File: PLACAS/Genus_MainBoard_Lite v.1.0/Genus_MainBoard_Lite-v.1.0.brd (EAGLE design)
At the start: 70 x 86 mm, 60 parts, among them U1 FT232RLSSOP, U2 MP2307DN-LF-Z, X1 53398-06, X15 JST-XH-05-PIN-LONG-PAD, X2 JST-XH-08-PIN-ROUND-PAD, X3 USB-SMD-NS, X5 53398-06

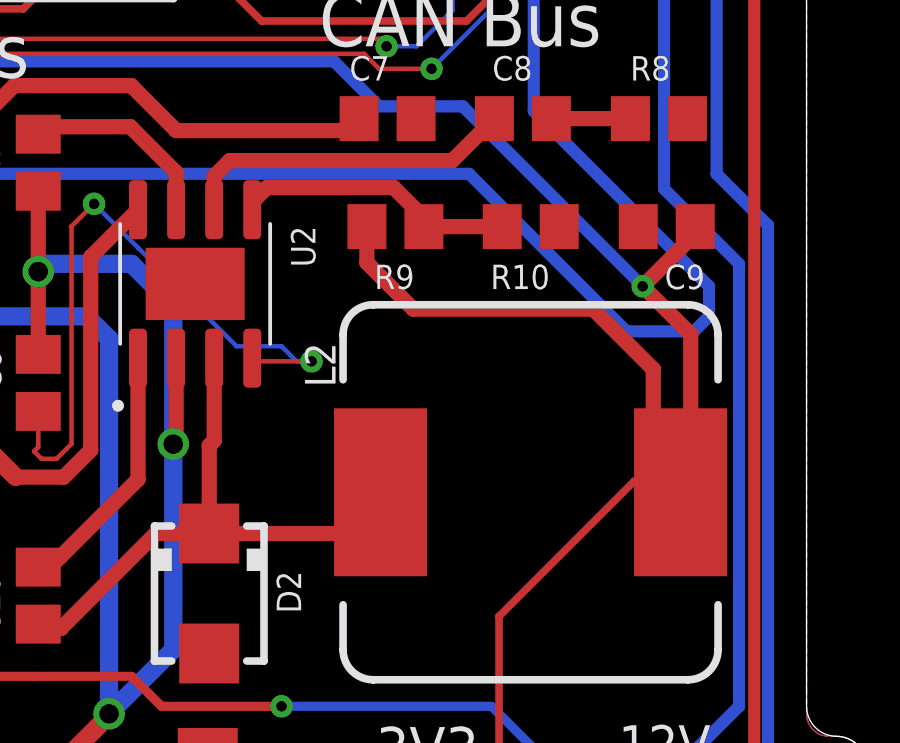
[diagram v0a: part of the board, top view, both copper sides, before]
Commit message: Add files via upload
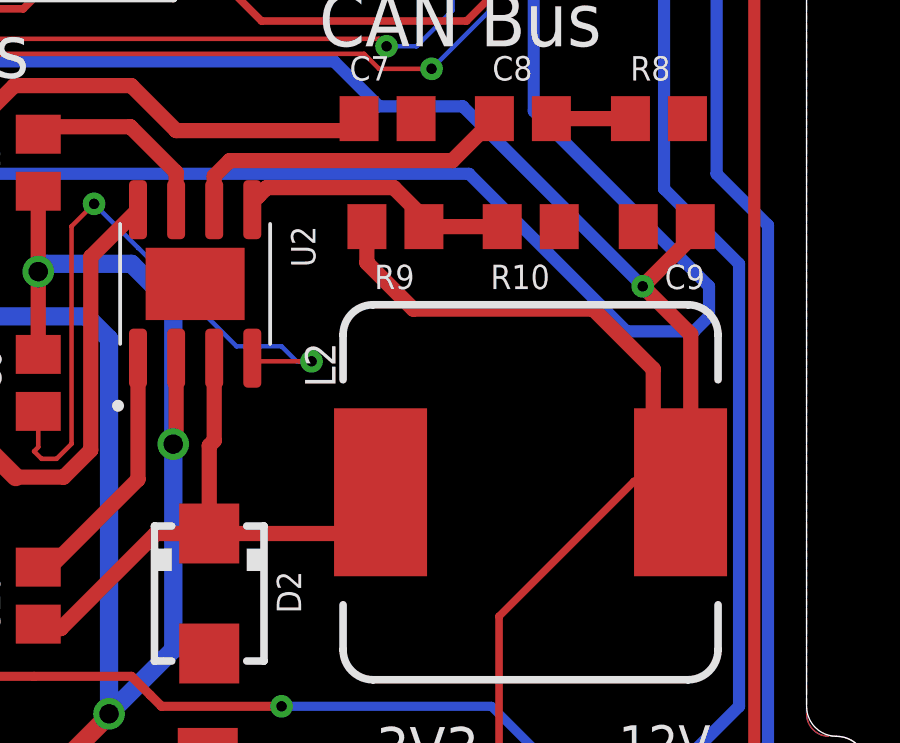
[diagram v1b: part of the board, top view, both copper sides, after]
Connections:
- new net BOOT: SLOT-1.A13, SLOT-2.A13
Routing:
- net OUT_3V3: track 86.4 -> 90.7 mm
- net N$12: track 22.1 -> 23.4 mm
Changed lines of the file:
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@@
 <?xml version="1.0" encoding="utf-8"?>
 <!DOCTYPE eagle SYSTEM "eagle.dtd">
-<eagle version="9.5.2">
+<eagle version="9.4.2">
 <drawing>
 <settings>
-<setting alwaysvectorfont="no"/>
+<setting alwaysvectorfont="yes"/>
 <setting verticaltext="up"/>
 </settings>
@@
 <contactref element="C10" pad="1"/>
 <contactref element="D2" pad="C"/>
-<wire x1="53.72" y1="26.73" x2="53.085" y2="26.095" width="0.6096" layer="1"/>
+<wire x1="53.085" y1="26.095" x2="53.72" y2="26.73" width="0.6096" layer="1"/>
 <wire x1="53.165" y1="27.5" x2="53.8" y2="28.135" width="0.508" layer="1"/>
 <wire x1="42.39" y1="23.74" x2="42.54" y2="23.59" width="0.508" layer="1"/>
@@
 <wire x1="46.31" y1="26.76" x2="48.09" y2="26.76" width="0.508" layer="1"/>
 <wire x1="43.14" y1="23.59" x2="46.31" y2="26.76" width="0.508" layer="1"/>
-<wire x1="48.09" y1="26.76" x2="53.66" y2="26.76" width="0.508" layer="1"/>
-<wire x1="53.66" y1="26.76" x2="54.14" y2="27.24" width="0.508" layer="1"/>
-<wire x1="53.8" y1="27.58" x2="53.8" y2="28.135" width="0.508" layer="1"/>
-<wire x1="54.14" y1="27.24" x2="53.8" y2="27.58" width="0.508" layer="1"/>
+<wire x1="52.5" y1="26.76" x2="48.09" y2="26.76" width="0.508" layer="1"/>
 <wire x1="48.09" y1="26.76" x2="48.09" y2="29.69" width="0.508" layer="1"/>
 <wire x1="48.255" y1="29.855" x2="48.255" y2="32.605" width="0.508" layer="1"/>
 <wire x1="48.09" y1="29.69" x2="48.255" y2="29.855" width="0.508" layer="1"/>
-<wire x1="53.165" y1="27.5" x2="53.72" y2="26.73" width="0" layer="19" extent="1-1"/>
+<wire x1="53.8" y1="28.135" x2="53.8" y2="28.06" width="0.1524" layer="1"/>
+<wire x1="53.8" y1="28.06" x2="52.5" y2="26.76" width="0.1524" layer="1"/>
+<wire x1="53.8" y1="28.135" x2="53.8" y2="26.81" width="0.1524" layer="1"/>
+<wire x1="53.8" y1="26.81" x2="53.085" y2="26.095" width="0.1524" layer="1"/>
 </signal>
 <signal name="N$13">
@@
 <contactref element="U2" pad="5"/>
 <wire x1="57.855" y1="36.99" x2="55.245" y2="36.99" width="0.508" layer="1"/>
-<wire x1="50.01" y1="38.29" x2="49.525" y2="37.805" width="0.508" layer="1"/>
+<wire x1="50.01" y1="38.29" x2="49.735" y2="38.015" width="0.508" layer="1"/>
+<wire x1="49.735" y1="38.015" x2="49.525" y2="37.805" width="0.508" layer="1"/>
 <wire x1="50.01" y1="38.29" x2="54.24" y2="38.29" width="0.508" layer="1"/>
 <wire x1="54.24" y1="38.29" x2="55.245" y2="37.285" width="0.508" layer="1"/>
 <wire x1="55.245" y1="37.285" x2="55.245" y2="36.99" width="0.508" layer="1"/>
-<wire x1="49.525" y1="37.805" x2="49.525" y2="37.555" width="0" layer="19" extent="1-1"/>
+<wire x1="49.525" y1="37.555" x2="49.525" y2="37.805" width="0.1524" layer="1"/>
 </signal>
 <signal name="OUT_3V3">
@@
 <wire x1="64.29" y1="36.75" x2="62.54" y2="35" width="0.508" layer="1"/>
 <wire x1="62.54" y1="35" x2="64.14" y2="33.4" width="0.508" layer="1"/>
-<wire x1="64.14" y1="33.4" x2="64.14" y2="29.49" width="0.508" layer="1"/>
+<wire x1="64.14" y1="29.49" x2="64.14" y2="30" width="0.508" layer="1"/>
+<wire x1="64.14" y1="30" x2="64.14" y2="33.4" width="0.508" layer="1"/>
 <wire x1="53.345" y1="36.99" x2="53.345" y2="35.785" width="0.508" layer="1"/>
 <wire x1="54.89" y1="34.24" x2="60.89" y2="34.24" width="0.508" layer="1"/>
 <wire x1="60.89" y1="34.24" x2="62.89" y2="32.24" width="0.508" layer="1"/>
-<wire x1="62.89" y1="32.24" x2="62.89" y2="30.74" width="0.508" layer="1"/>
+<wire x1="62.89" y1="32.24" x2="62.89" y2="29.64" width="0.508" layer="1"/>
 <wire x1="53.345" y1="35.785" x2="54.89" y2="34.24" width="0.508" layer="1"/>
 <contactref element="F3" pad="2"/>
@@
 <wire x1="57.75" y1="18.97" x2="57.75" y2="24" width="0.254" layer="1"/>
 <wire x1="57.75" y1="24" x2="62.25" y2="28.5" width="0.254" layer="1"/>
-<wire x1="62.25" y1="28.5" x2="64.25" y2="28.5" width="0.254" layer="1"/>
-<wire x1="64.25" y1="28.5" x2="63.885" y2="28.135" width="0.254" layer="1"/>
-<wire x1="63.885" y1="28.135" x2="63.8" y2="28.135" width="0.254" layer="1"/>
+<wire x1="63.5" y1="28.5" x2="62.25" y2="28.5" width="0.254" layer="1"/>
 <wire x1="29.79" y1="40.02" x2="29.79" y2="41.52" width="0.4064" layer="1"/>
 <wire x1="28" y1="42.5" x2="28.81" y2="42.5" width="0.4064" layer="1"/>
@@
 <wire x1="56.54" y1="41" x2="62.54" y2="35" width="0.4064" layer="16"/>
 <via x="62.54" y="35" extent="1-16" drill="0.35"/>
-<wire x1="64.14" y1="29.49" x2="62.89" y2="30.74" width="0" layer="19" extent="1-1"/>
-<wire x1="63.8" y1="28.135" x2="64.14" y2="29.49" width="0" layer="19" extent="1-1"/>
+<wire x1="62.89" y1="29.64" x2="62.75" y2="29.5" width="0.508" layer="1"/>
+<wire x1="63.8" y1="28.135" x2="62.89" y2="29.045" width="0.1524" layer="1"/>
+<wire x1="62.89" y1="29.045" x2="62.89" y2="29.64" width="0.1524" layer="1"/>
+<wire x1="63.8" y1="28.135" x2="63.5" y2="28.435" width="0.3048" layer="1"/>
+<wire x1="63.5" y1="28.435" x2="63.5" y2="28.5" width="0.3048" layer="1"/>
+<wire x1="63.8" y1="28.135" x2="63.8" y2="29.66" width="0.3048" layer="1"/>
+<wire x1="63.8" y1="29.66" x2="64.14" y2="30" width="0.3048" layer="1"/>
 </signal>
 <signal name="N$14">
@@
 <wire x1="64.05" y1="14.845" x2="63.95" y2="14.745" width="0.4064" layer="1"/>
 </signal>
+<signal name="BOOT">
+<contactref element="SLOT-2" pad="A13"/>
+<contactref element="SLOT-1" pad="A13"/>
+<wire x1="46.34" y1="58.01" x2="46.34" y2="73.01" width="0" layer="19" extent="1-1"/>
+</signal>
 </signals>
